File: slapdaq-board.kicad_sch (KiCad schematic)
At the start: 21 parts, among them J1 12-24V POWER IN, U1 LMR51430 - 5V REG, U2 LMR51430 - 3.3V REG

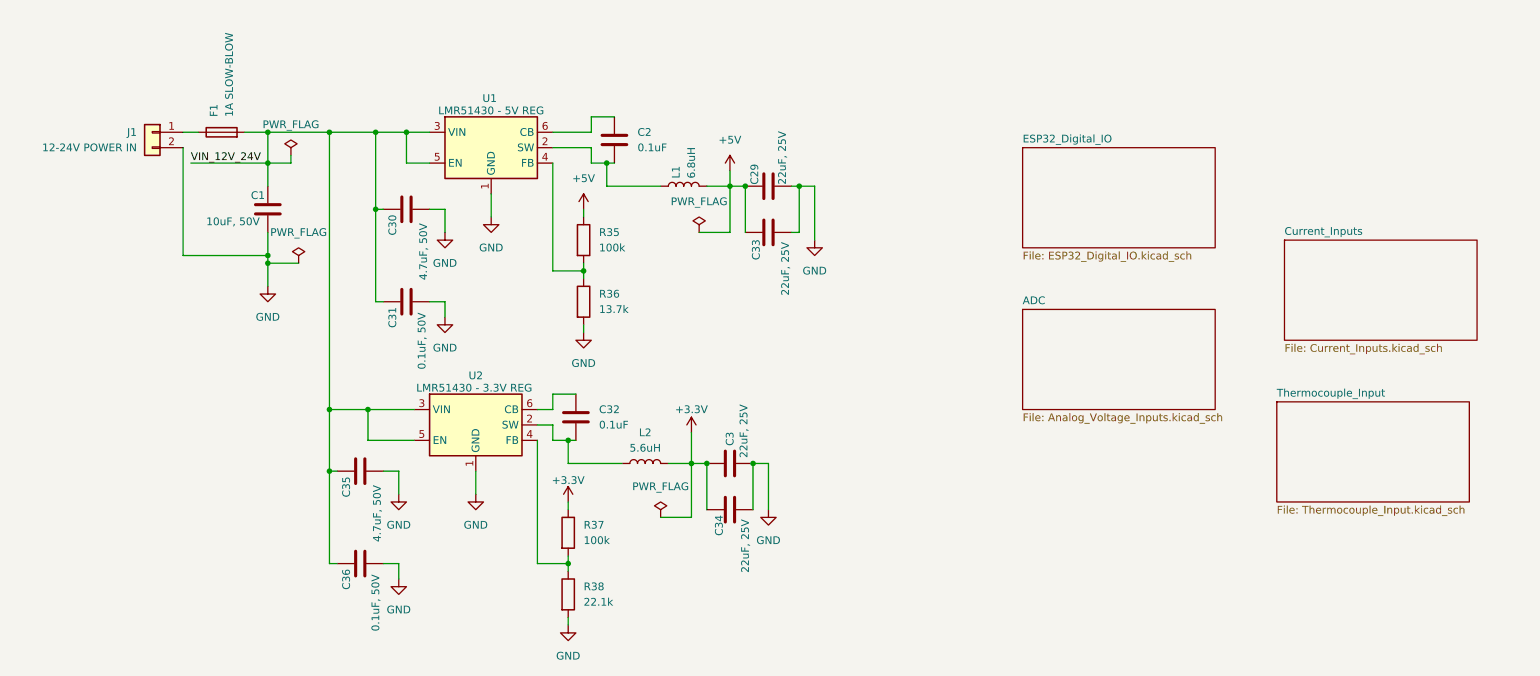
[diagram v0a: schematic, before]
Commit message: Grayson changes 9/11/26
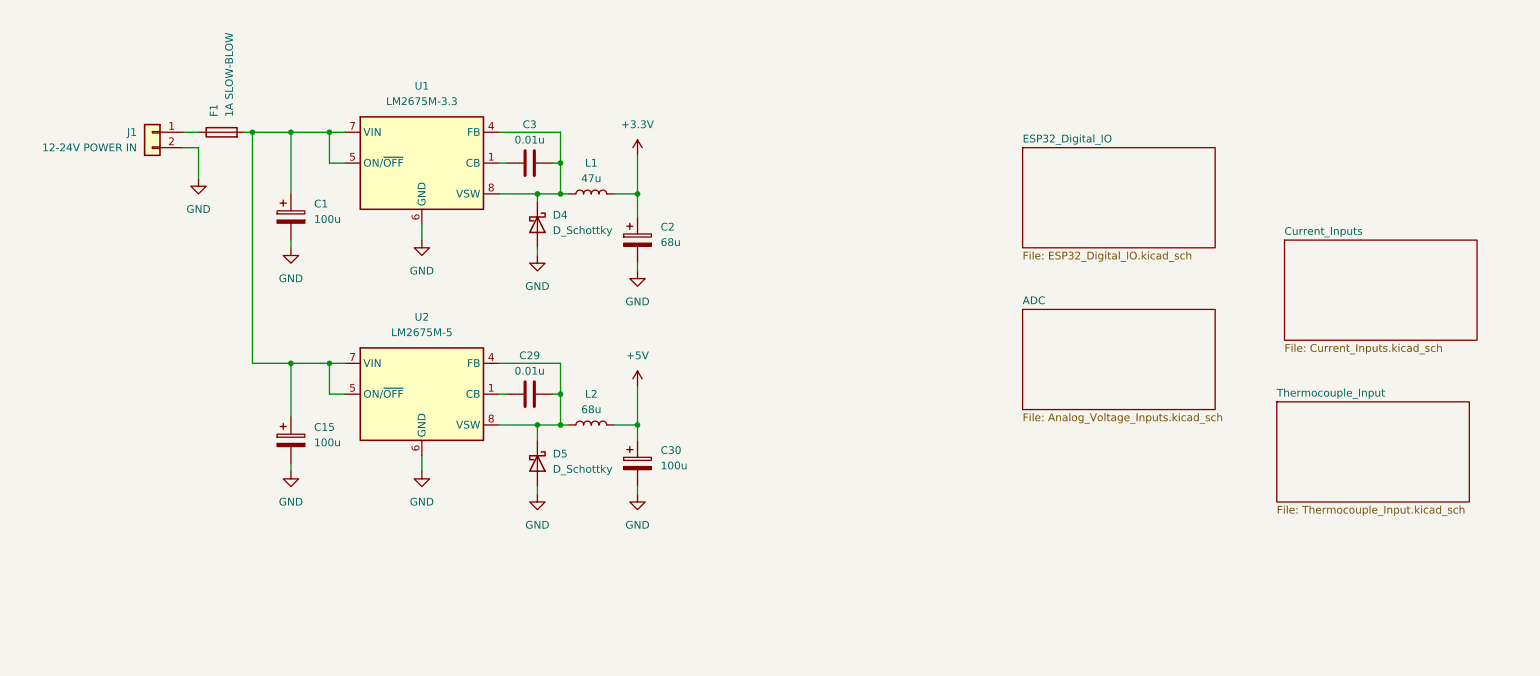
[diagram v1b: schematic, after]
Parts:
- removed C1: 10uF, 50V, symbol Device:C
- removed C2, C32: 0.1uF, symbol Device:C
- removed C30, C35: 4.7uF, 50V, symbol Device:C
- removed C31, C36: 0.1uF, 50V, symbol Device:C
- removed C33, C34: 22uF, 25V, symbol Device:C
- removed R35, R37: 100k, symbol Device:R
- removed R36: 13.7k, symbol Device:R
- removed R38: 22.1k, symbol Device:R
- removed U1: LMR51430 - 5V REG, Package_TO_SOT_SMD:SOT-23-6, symbol Regulator_Switching:LMR51430
- removed U2: LMR51430 - 3.3V REG, Package_TO_SOT_SMD:SOT-23-6, symbol Regulator_Switching:LMR51430
- added C1, C15, C30: 100u, symbol Device:C_Polarized
- added C2: 68u, symbol Device:C_Polarized
- added D4, D5: D_Schottky, symbol Device:D_Schottky
- added U1: LM2675M-3.3, Package_SO:SOIC-8_3.9x4.9mm_P1.27mm, symbol Regulator_Switching:LM2675M-3.3
- added U2: LM2675M-5, Package_SO:SOIC-8_3.9x4.9mm_P1.27mm, symbol Regulator_Switching:LM2675M-5
- C29, C3: value 22uF, 25V -> 0.01u
- L1: value 6.8uH -> 47u; footprint Package_TO_SOT_SMD:SOT-23-6 -> (none)
- L2: value 5.6uH -> 68u; footprint Package_TO_SOT_SMD:SOT-23-6 -> (none)
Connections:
- net +3.3V: now also L1.2, C2.1; no longer C3.1, L2.2
- net +5V: now also L2.2, C30.1; no longer C29.1, L1.2
- net GND: now also C1.2, C15.2, C2.2, C30.2, D4.2 (A), D5.2 (A), U1.6 (GND), U2.6 (GND); no longer C29.2, C3.2
- net at L2.1: now also C29.2, D5.1 (K), U2.4 (FB), U2.8 (VSW)
- net at L1.1: now also C3.2, D4.1 (K), U1.4 (FB), U1.8 (VSW)
- net VIN_12V_24V: no longer names the net of F1.2
- net VIN_12V_24V: now also C1.1, C15.1, U1.5 (ON/~{OFF}), U1.7 (VIN), U2.5 (ON/~{OFF}), U2.7 (VIN)
- new net: C3.1, U1.1 (CB)
- new net: C29.1, U2.1 (CB)
